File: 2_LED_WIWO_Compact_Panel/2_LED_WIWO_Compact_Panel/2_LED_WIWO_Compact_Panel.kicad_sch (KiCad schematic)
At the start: 7 parts, among them U1 NE555DR-EV, U2 XL1509, U3 NE555DR-EV, U4 MP24833-AGN-Z, U5 AP2210N-5.0TRG1

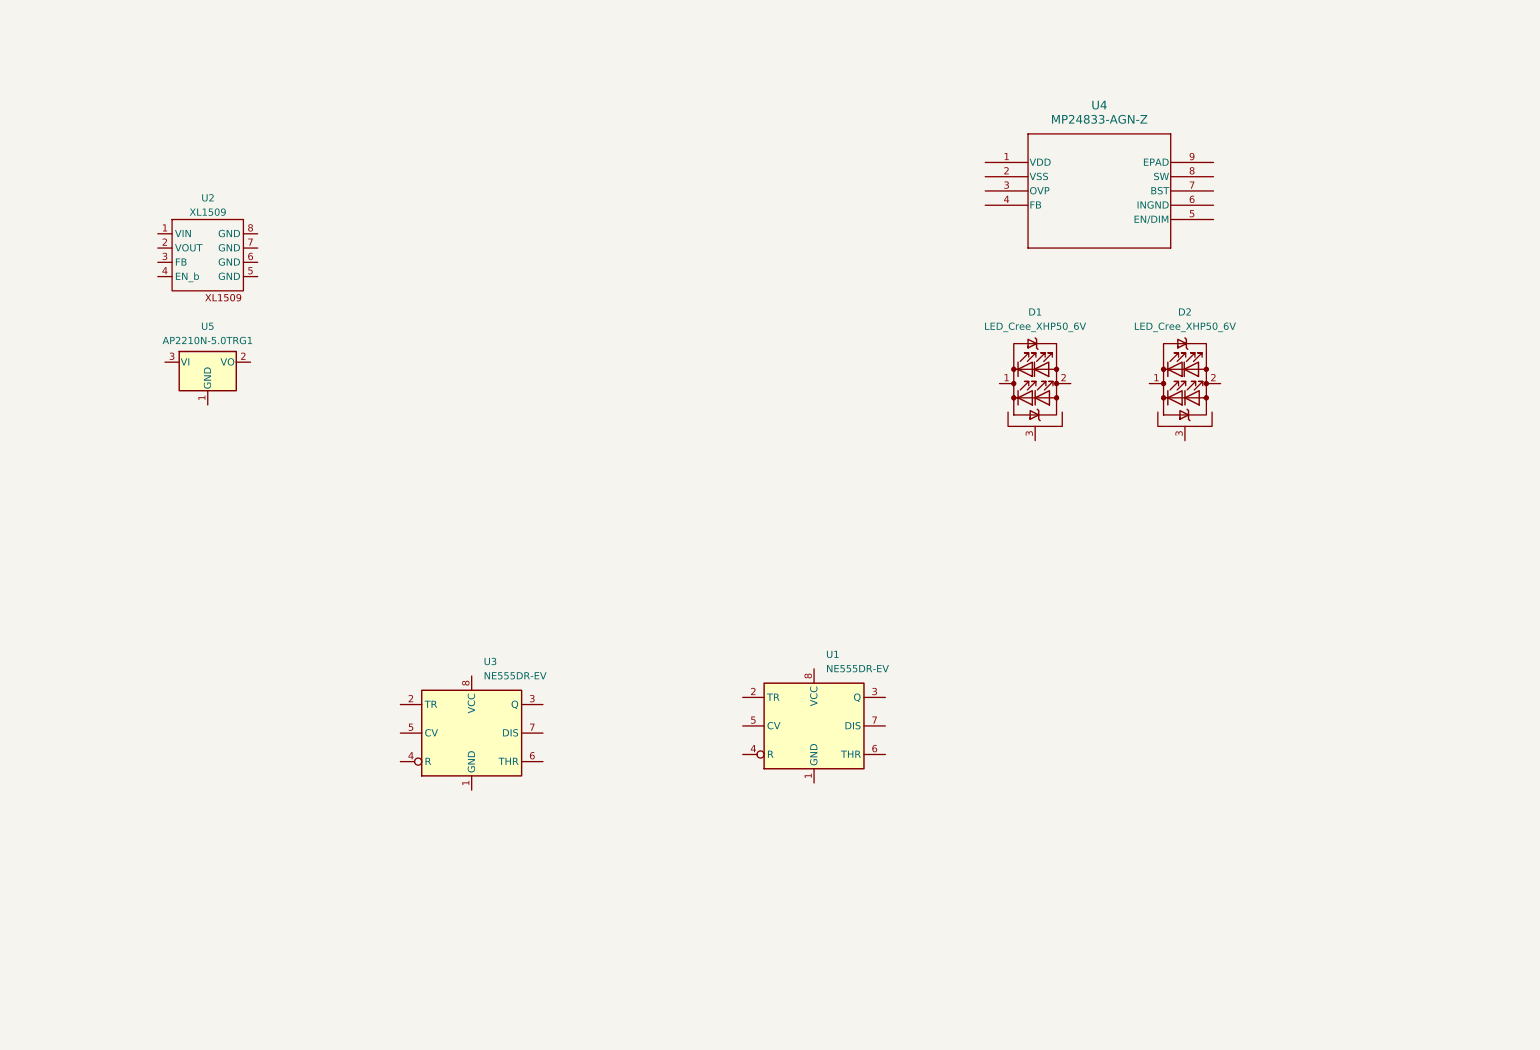
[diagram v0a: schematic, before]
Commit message: finished v1 schem and moving to layout
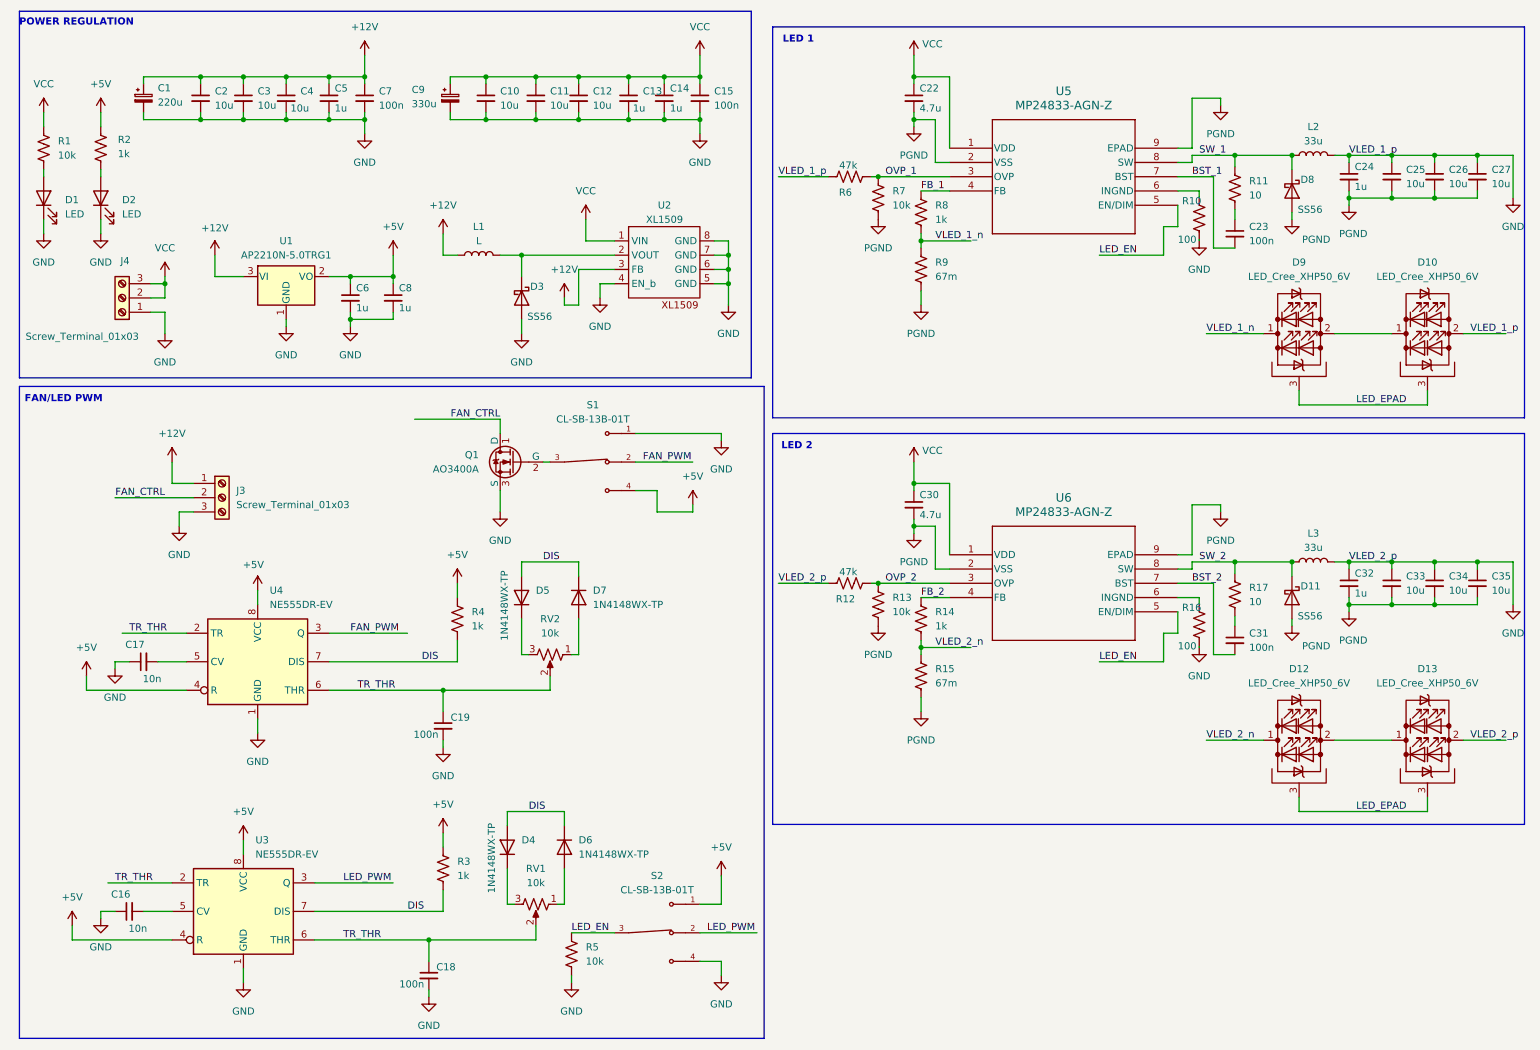
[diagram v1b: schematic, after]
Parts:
- removed U1: NE555DR-EV, Package_SO:SOIC-8_3.9x4.9mm_P1.27mm, symbol Timer:NE555D
- added C1: 220u, 12V_Buck_Footprints:CAP_6.3 X 7.7_PAN, symbol Device:C_Polarized_Small
- added C10, C11, C12, C2, C25, C26, C27, C3, C33, C34, C35, C4: 10u, Capacitor_SMD:C_0603_1608Metric_Pad1.08x0.95mm_HandSolder, symbol Device:C_Small
- added C13, C14, C5, C6, C8: 1u, Capacitor_SMD:C_0402_1005Metric_Pad0.74x0.62mm_HandSolder, symbol Device:C_Small
- added C15, C7: 100n, Capacitor_SMD:C_0201_0603Metric_Pad0.64x0.40mm_HandSolder, symbol Device:C_Small
- added C16, C17: 10n, Resistor_SMD:R_0201_0603Metric_Pad0.64x0.40mm_HandSolder, symbol Device:C_Small
- added C18, C19: 100n, Resistor_SMD:R_0402_1005Metric_Pad0.72x0.64mm_HandSolder, symbol Device:C_Small
- added C22, C30: 4.7u, Capacitor_SMD:C_0603_1608Metric_Pad1.08x0.95mm_HandSolder, symbol Device:C_Small
- added C23, C31: 100n, Capacitor_SMD:C_0603_1608Metric_Pad1.08x0.95mm_HandSolder, symbol Device:C_Small
- added C24, C32: 1u, Capacitor_SMD:C_0603_1608Metric_Pad1.08x0.95mm_HandSolder, symbol Device:C_Small
- added C9: 330u, compact_LED_Panel_footprints:CAPAE1030X1050N, symbol Device:C_Polarized_Small
- added D1, D2: LED, LED_SMD:LED_0603_1608Metric_Pad1.05x0.95mm_HandSolder, symbol Device:LED
- added D11, D3, D8: SS56, Diode_SMD:D_SMA_Handsoldering, symbol Device:D_Schottky
- added D12, D13: LED_Cree_XHP50_6V, LED_SMD:LED_Cree-XHP50_6V, symbol LED:LED_Cree_XHP50_6V
- added D4, D5, D6, D7: 1N4148WX-TP, Diode_SMD:D_SOD-323_HandSoldering, symbol Device:D
- added J3, J4: Screw_Terminal_01x03, TerminalBlock:TerminalBlock_MaiXu_MX126-5.0-03P_1x03_P5.00mm, symbol Connector:Screw_Terminal_01x03
- added L1: L, 12V_Buck_Footprints:CDRH127L125NP-680MC, symbol Device:L
- added L2, L3: 33u, 12V_Buck_Footprints:IND_SRP1265A-330M, symbol Device:L
- added Q1: AO3400A, Package_TO_SOT_SMD:SOT-23_Handsoldering, symbol Simulation_SPICE:NMOS
- added R1, R13, R5, R7: 10k, Resistor_SMD:R_0402_1005Metric_Pad0.72x0.64mm_HandSolder, symbol Device:R_US
- added R10, R16: 100, Resistor_SMD:R_0603_1608Metric_Pad0.98x0.95mm_HandSolder, symbol Device:R_US
- added R11, R17: 10, Resistor_SMD:R_0603_1608Metric_Pad0.98x0.95mm_HandSolder, symbol Device:R_US
- added R12, R6: 47k, Resistor_SMD:R_0402_1005Metric_Pad0.72x0.64mm_HandSolder, symbol Device:R_US
- added R14, R2, R3, R4, R8: 1k, Resistor_SMD:R_0402_1005Metric_Pad0.72x0.64mm_HandSolder, symbol Device:R_US
- added R15, R9: 67m, Resistor_SMD:R_2512_6332Metric_Pad1.40x3.35mm_HandSolder, symbol Device:R_US
- added RV1, RV2: 10k, compact_LED_Panel_footprints:PTV09A-4015F-B104_BRN, symbol Device:R_Potentiometer_US
- added S1, S2: CL-SB-13B-01T, compact_LED_Panel_footprints:SW_CL-SB-13B-01T, symbol CL-SB-13B-01T:CL-SB-13B-01T
- added U4: NE555DR-EV, Package_SO:SOIC-8_3.9x4.9mm_P1.27mm, symbol Timer:NE555D
- added U6: MP24833-AGN-Z, Package_SO:SOIC-8-1EP_3.9x4.9mm_P1.27mm_EP2.514x3.2mm_ThermalVias, symbol MP24833-AGN-Z:MP24833-AGN-Z
- renumbered D2 to D10, D1 to D9, U5 to U1, U4 to U5
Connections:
- net VCC: now reaches U2.1 (VIN)
- net VCC: now also U5.1 (VDD), C10.1, C11.1, C12.1, C13.1, C14.1, C15.1, C22.1, C30.1, C9.1, J4.2 (Pin_2), J4.3 (Pin_3), R1.1, U6.1 (VDD)
- net at U2.2 (VOUT): now also D3.1 (K), L1.2
- net +12V: now reaches U2.3 (FB)
- net +12V: now also U1.3 (VI), C1.1, C2.1, C3.1, C4.1, C5.1, C7.1, J3.1 (Pin_1), L1.1
- net GND: now reaches U2.4 (EN_b)
- net GND: now also D10.2 (A), U1.1 (GND), U2.5 (GND), U2.6 (GND), U2.7 (GND), U2.8 (GND), U3.1 (GND), C1.2, C10.2, C11.2, C12.2, C13.2, C14.2, C15.2, C16.1, C17.1, C18.2, C19.2, C2.2, C24.1, C25.1, C26.1, C27.1, C3.2, C32.1, C33.1, C34.1, C35.1, C4.2, C5.2, C6.2, C7.2, C8.2, C9.2, D1.1 (K), D13.2 (A), D2.1 (K), D3.2 (A), J3.3 (Pin_3), J4.1 (Pin_1), L2.2, L3.2, Q1.3 (S), R10.2, R12.1, R16.2, R5.2, R6.1, S1.1, S2.4, U4.1 (GND)
- net VLED_1_n: now reaches D9.1 (K)
- net VLED_1_n: now also R8.2, R9.1
- net at D9.2 (A): now also D10.1 (K)
- net LED_EPAD: now reaches D9.3 (PAD)
- net LED_EPAD: now also D10.3 (PAD), D12.3 (PAD), D13.3 (PAD)
- net +5V: now reaches U1.2 (VO)
- net +5V: now also U3.4 (R), U3.8 (VCC), C6.1, C8.1, R2.1, R3.1, R4.1, S1.4, S2.1, U4.4 (R), U4.8 (VCC)
- net TR_THR: now reaches U3.2 (TR)
- net TR_THR: now also U3.6 (THR), C18.1, C19.1, RV1.2, RV2.2, U4.2 (TR), U4.6 (THR)
- net LED_PWM: now reaches U3.3 (Q)
- net LED_PWM: now also S2.2
- net at U3.5 (CV): now also C16.2
- net DIS: now reaches U3.7 (DIS)
- net DIS: now also D4.2 (A), D5.2 (A), D6.1 (K), D7.1 (K), R3.2, R4.2, U4.7 (DIS)
- net PGND: now reaches U5.2 (VSS)
- net PGND: now also U5.9 (EPAD), C22.2, C24.2, C25.2, C26.2, C27.2, C30.2, C32.2, C33.2, C34.2, C35.2, D11.2 (A), D8.2 (A), R13.2, R15.2, R7.2, R9.2, U6.2 (VSS), U6.9 (EPAD)
- net OVP_1: now reaches U5.3 (OVP)
- net OVP_1: now also R6.2, R7.1
- net FB_1: now reaches U5.4 (FB)
- net FB_1: now also R8.1
- net LED_EN: now reaches U5.5 (EN/DIM)
- net LED_EN: now also R5.1, S2.3, U6.5 (EN/DIM)
- net at U5.6 (INGND): now also R10.1
- net BST_1: now reaches U5.7 (BST)
- net BST_1: now also C23.2
- net SW_1: now reaches U5.8 (SW)
- net SW_1: now also D8.1 (K), L2.1, R11.1
- new net: Q1.2 (G), S1.3
- new net: C31.1, R17.2
- new net: C23.1, R11.2
- new net: D2.2 (A), R2.2
- new net: R16.1, U6.6 (INGND)
- new net: C17.2, U4.5 (CV)
- new net: D12.2 (A), D13.1 (K)
- new net: D4.1 (K), RV1.3
- new net: D6.2 (A), RV1.1
- new net: D7.2 (A), RV2.1
- new net: D5.1 (K), RV2.3
- new net: D1.2 (A), R1.2
- new net BST_2: C31.2, U6.7 (BST)
- new net FAN_CTRL: J3.2 (Pin_2), Q1.1 (D)
- new net FAN_PWM: S1.2, U4.3 (Q)
- new net FB_2: R14.1, U6.4 (FB)
- new net OVP_2: R12.2, R13.1, U6.3 (OVP)
- new net SW_2: D11.1 (K), L3.1, R17.1, U6.8 (SW)
- new net VLED_2_n: D12.1 (K), R14.2, R15.1
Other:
- note added: "FAN/LED PWM"
- note added: "LED 1"
- note added: "LED 2"
- note added: "POWER REGULATION"
- moved on the sheet: D10, D9, U1, U2, U3, U5
